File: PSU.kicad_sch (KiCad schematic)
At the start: 3 parts, among them U2 MCP1754ST-3302E/MB

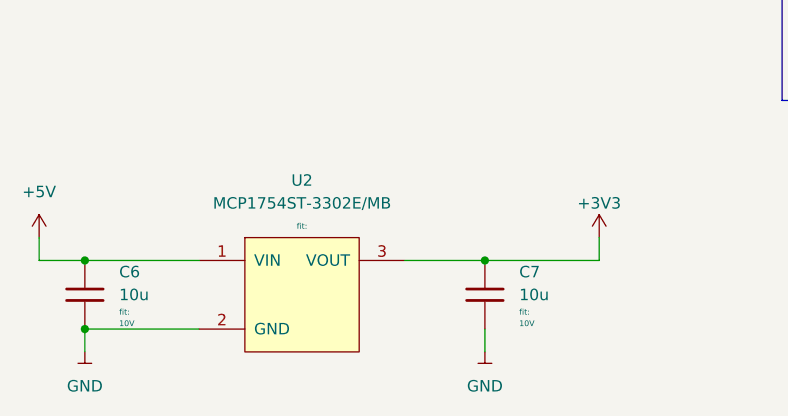
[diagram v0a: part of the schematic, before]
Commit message: gsi-v1
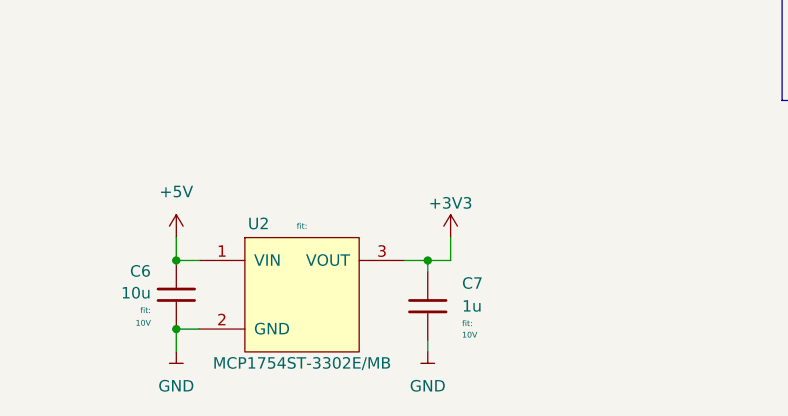
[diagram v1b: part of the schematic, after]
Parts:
- C6: note (none) -> stock
- C7: value 10u_0805_X7R_10%_10V_-40C..125C_Chip-Capacitor -> 1u_0805_X7R_10%_10V_-40C..125C_Chip-Capacitor; DisplayValue 10u -> 1u; note (none) -> stock
- U2: digikey (none) -> MCP1754ST-3302E/MBCT-ND
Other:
- moved on the sheet: C6, C7

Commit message: ready for production
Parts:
- C6: value 10u_0805_X7R_10%_10V_-40C..125C_Chip-Capacitor -> 10u; footprint Capacitor_SMD:C_0805_2012Metric -> Capacitor_SMD:C_0603_1608Metric; note stock -> candlelight; now left out of the parts list
- C7: value 1u_0805_X7R_10%_10V_-40C..125C_Chip-Capacitor -> 1u; footprint Capacitor_SMD:C_0805_2012Metric -> Capacitor_SMD:C_0603_1608Metric; note stock -> candlelight; now left out of the parts list
- U2: note (none) -> candlelight
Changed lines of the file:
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@@
 		(unit 1)
 		(exclude_from_sim no)
-		(in_bom yes)
+		(in_bom no)
 		(on_board yes)
 		(dnp no)
@@
 			)
 		)
-		(property "Value" "1u_0805_X7R_10%_10V_-40C..125C_Chip-Capacitor"
+		(property "Value" "1u"
 			(at 158.115 99.06 0)
 			(effects
@@
 			)
 		)
-		(property "Footprint" "Capacitor_SMD:C_0805_2012Metric"
+		(property "Footprint" "Capacitor_SMD:C_0603_1608Metric"
 			(at 158.4452 100.33 0)
 			(effects
@@
 			)
 		)
-		(property "note" "stock"
+		(property "note" "candlelight"
 			(at 157.48 96.52 0)
 			(effects
@@
 		(unit 1)
 		(exclude_from_sim no)
-		(in_bom yes)
+		(in_bom no)
 		(on_board yes)
 		(dnp no)
@@
 			)
 		)
-		(property "Value" "10u_0805_X7R_10%_10V_-40C..125C_Chip-Capacitor"
+		(property "Value" "10u"
 			(at 128.905 97.79 0)
 			(effects
@@
 			)
 		)
-		(property "Footprint" "Capacitor_SMD:C_0805_2012Metric"
+		(property "Footprint" "Capacitor_SMD:C_0603_1608Metric"
 			(at 128.5748 99.06 0)
 			(effects
@@
 			)
 		)
-		(property "note" "stock"
+		(property "note" "candlelight"
 			(at 129.54 95.25 0)
 			(effects
@@
 			)
 		)
-		(property "note" ""
+		(property "note" "candlelight"
 			(at 143.51 95.25 0)
 			(effects
